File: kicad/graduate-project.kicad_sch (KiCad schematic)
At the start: 16 parts, among them J1 Power, J2 GY-9250, J3 HM-10, J4 Left Motor, J5 Right Motor, U1 NUCLEO-L432KC, U2 DRV8847PWP

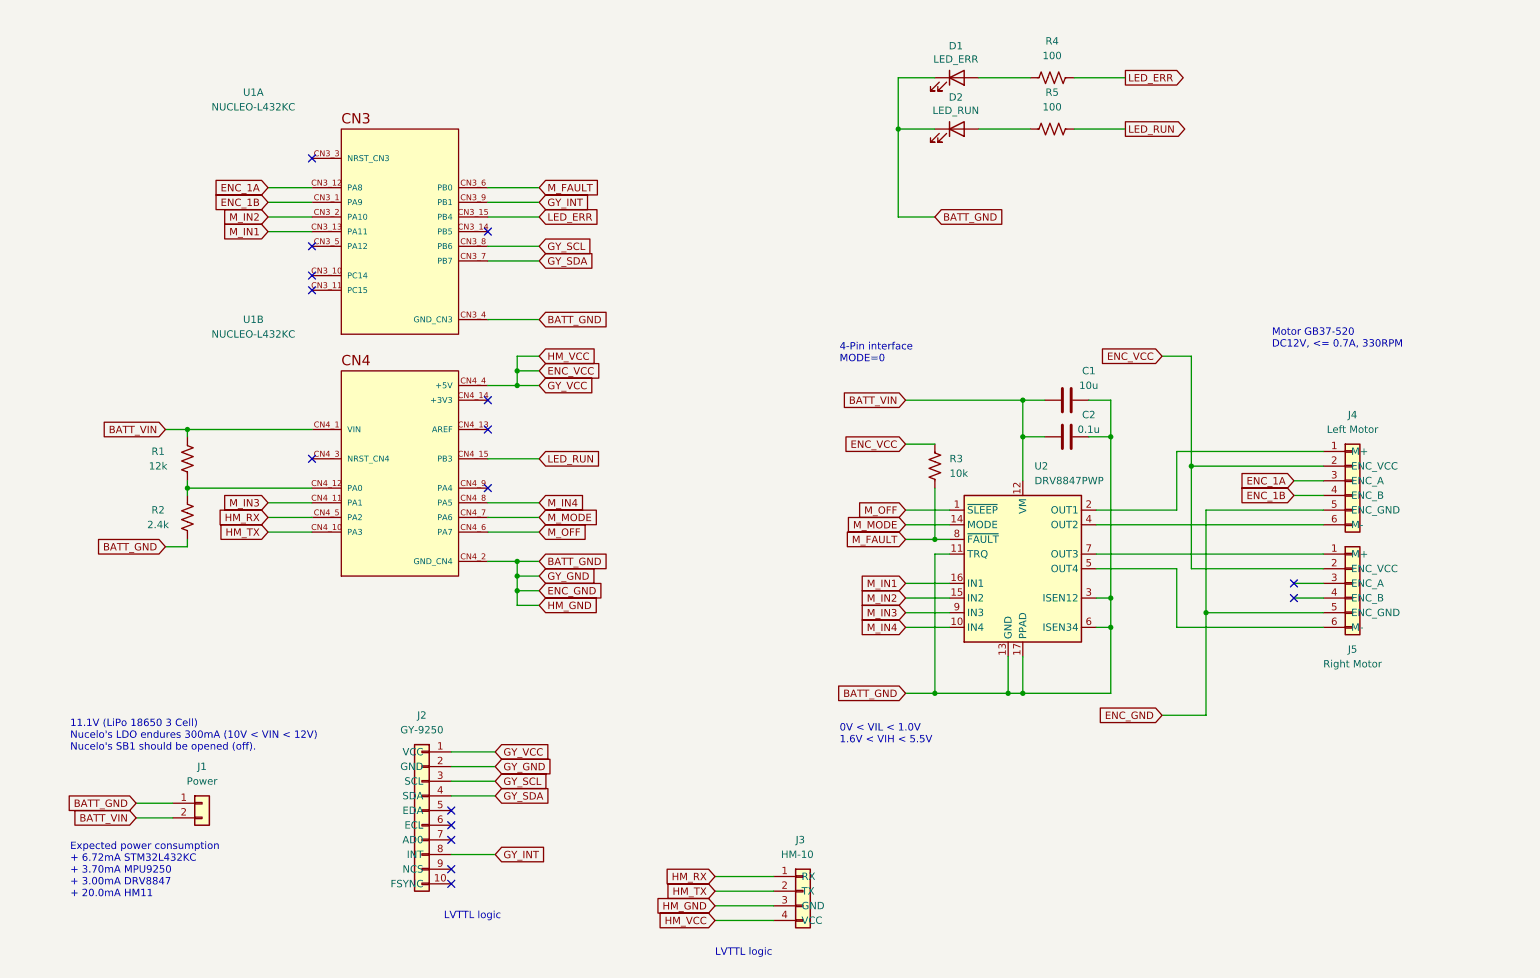
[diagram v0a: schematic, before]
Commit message: Update pdf plots
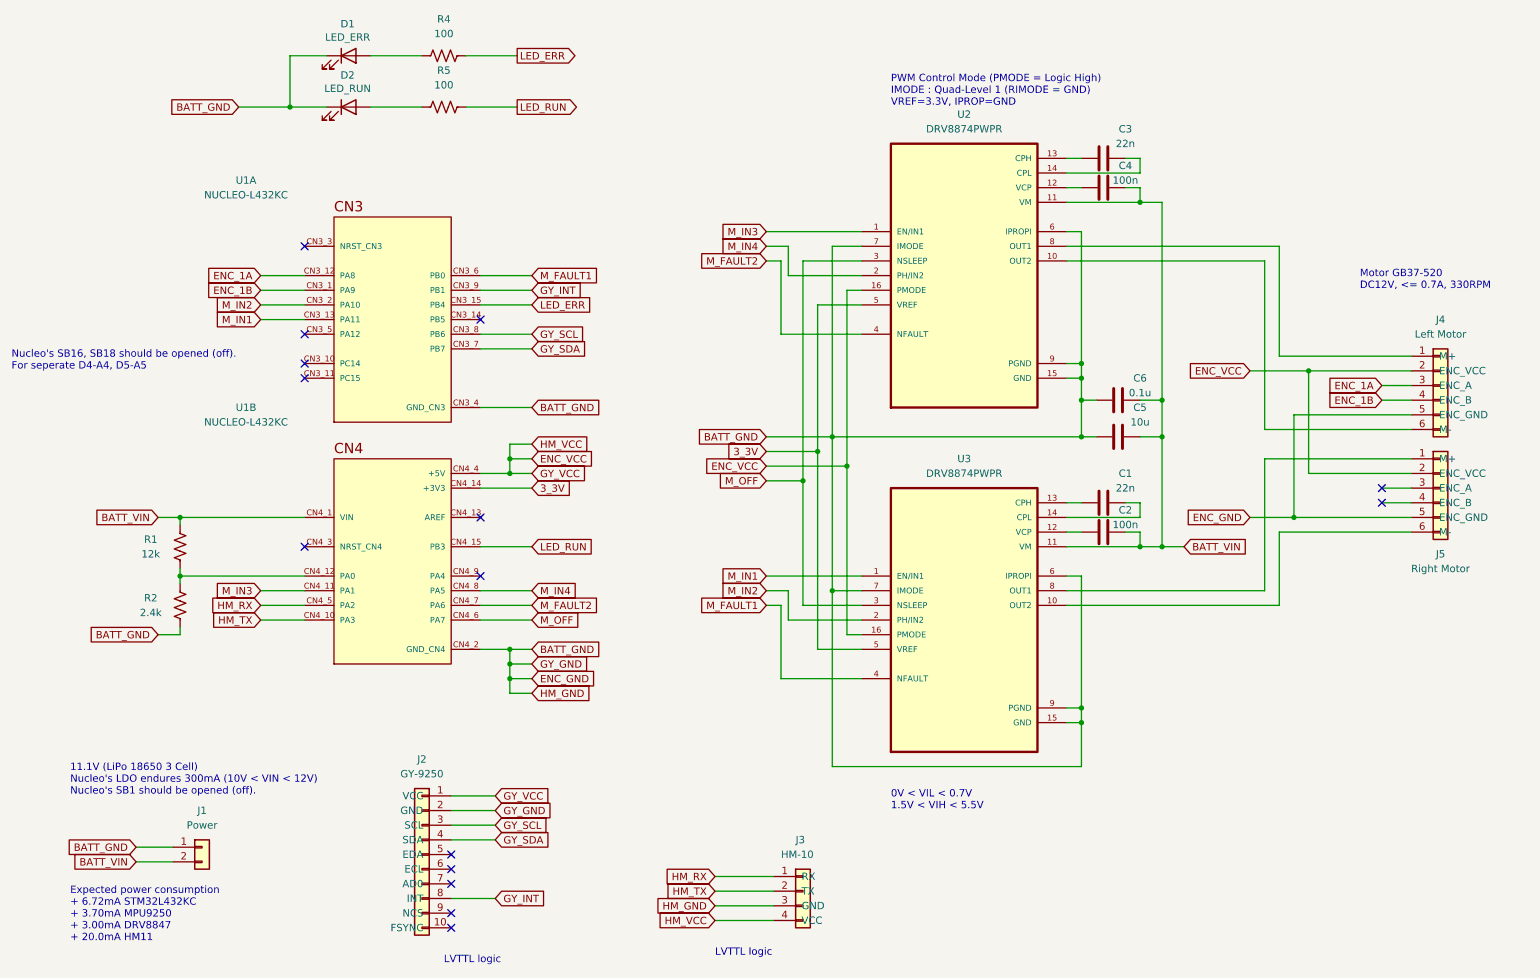
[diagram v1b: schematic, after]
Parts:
- removed R3: 10k, Resistor_SMD:R_0603_1608Metric, symbol Device:R_US
- removed U2: DRV8847PWP, Package_SO:HTSSOP-16-1EP_4.4x5mm_P0.65mm_EP3.4x5mm_Mask2.46x2.31mm_ThermalVias, symbol Driver_Motor:DRV8847PWP
- added C3: 22n, Capacitor_SMD:C_0603_1608Metric, symbol Device:C
- added C4: 100n, Capacitor_SMD:C_0603_1608Metric, symbol Device:C
- added C5: 10u, Capacitor_SMD:C_0603_1608Metric, symbol Device:C
- added C6: 0.1u, Capacitor_SMD:C_0603_1608Metric, symbol Device:C
- added U2, U3: DRV8874PWPR, SOP65P640X120-17N, symbol DRV8874PWPR:DRV8874PWPR
- C1: value 10u -> 22n; Temperature (none) -> X5R
- C2: value 0.1u -> 100n; Temperature (none) -> X5R
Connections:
- net BATT_GND: now also C5.1, C6.1, U2.15 (GND), U2.6 (IPROPI), U2.7 (IMODE), U2.9 (PGND), U3.15 (GND), U3.6 (IPROPI), U3.7 (IMODE), U3.9 (PGND); no longer C1.2, C2.2
- net BATT_VIN: now also C2.2, C4.2, C5.2, C6.2, U2.11 (VM), U3.11 (VM); no longer C1.1, C2.1
- net ENC_VCC: now also U2.16 (PMODE), U3.16 (PMODE)
- net M_IN1: now also U3.1 (EN/IN1)
- net M_IN2: now also U3.2 (PH/IN2)
- net M_IN3: now also U2.1 (EN/IN1)
- net M_IN4: now also U2.2 (PH/IN2)
- net M_OFF: now also U2.3 (NSLEEP), U3.3 (NSLEEP)
- net at J4.1 (M+): now also U2.8 (OUT1)
- net at J4.6 (M-): now also U2.10 (OUT2)
- net at J5.6 (M-): now also U3.10 (OUT2)
- net at J5.1 (M+): now also U3.8 (OUT1)
- net 3_3V: now reaches U1.CN4_14 (+3V3)
- net 3_3V: now also U2.5 (VREF), U3.5 (VREF)
- net M_FAULT renamed M_FAULT1
- net M_FAULT1: now also U3.4 (NFAULT)
- net M_MODE renamed M_FAULT2
- net M_FAULT2: now also U2.4 (NFAULT)
- new net: C4.1, U2.12 (VCP)
- new net: C3.1, U2.13 (CPH)
- new net: C3.2, U2.14 (CPL)
- new net: C1.1, U3.13 (CPH)
- new net: C1.2, U3.14 (CPL)
- new net: C2.1, U3.12 (VCP)
- no-connect marks 16 -> 15
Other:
- note added: "0V < VIL < 0.7V 1.5V < VIH < 5.5V"
- note added: "11.1V (LiPo 18650 3 Cell) Nucleo's LDO endures 300mA (10V < VIN < 12V) Nucleo's SB1 should be opened (off)."
- note added: "Nucleo's SB16, SB18 should be opened (off). For seperate D4-A4, D5-A5"
- note added: "PWM Control Mode (PMODE = Logic High) IMODE : Quad-Level 1 (RIMODE = GND) VREF=3.3V, IPROP=GND"
- note removed: "0V < VIL < 1.0V 1.6V < VIH < 5.5V"
- note removed: "11.1V (LiPo 18650 3 Cell) Nucelo's LDO endures 300mA (10V < VIN < 12V) Nucelo's SB1 should be opened (off)."
- note removed: "4-Pin interface MODE=0"
- moved on the sheet: C1, C2, D1, D2, J1, J2, J4, J5, R1, R2, R4, R5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
